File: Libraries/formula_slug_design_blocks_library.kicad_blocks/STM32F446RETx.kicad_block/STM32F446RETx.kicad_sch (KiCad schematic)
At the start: 18 parts

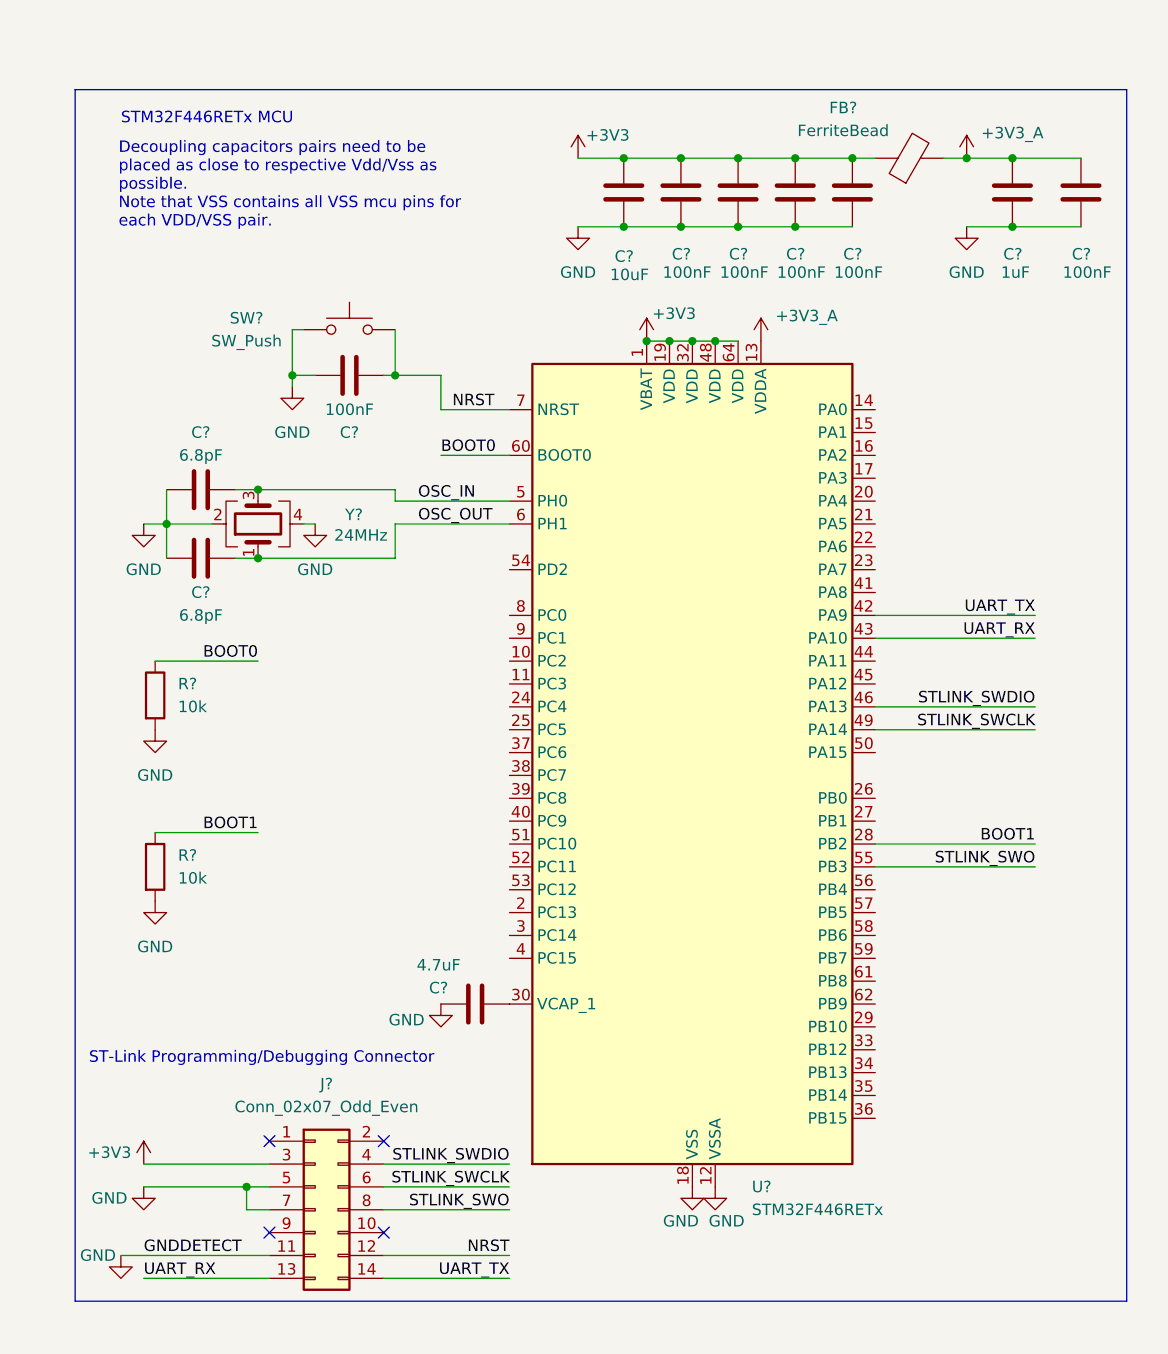
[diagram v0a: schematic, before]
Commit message: Fix issues
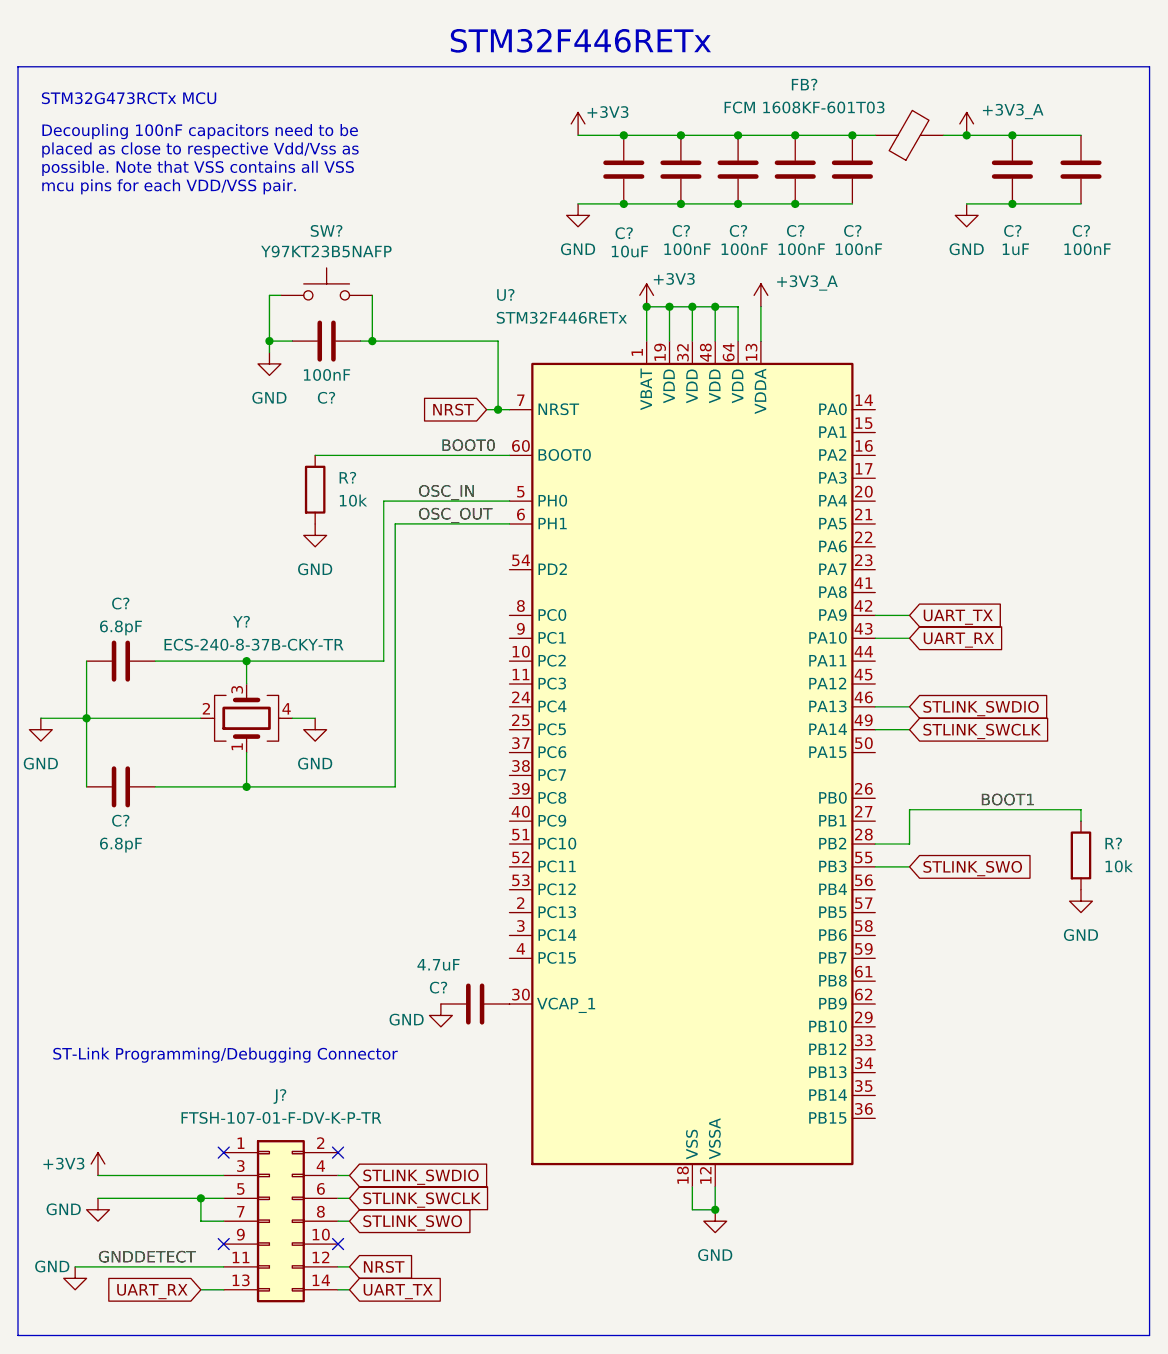
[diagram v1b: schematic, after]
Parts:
- removed C? (x2): 6.8pF, Capacitor_SMD:C_0805_2012Metric_Pad1.18x1.45mm_HandSolder, symbol Device:C
- removed C?: 100nF, Capacitor_SMD:C_0805_2012Metric_Pad1.18x1.45mm_HandSolder, symbol Device:C
- removed J?: Conn_02x07_Odd_Even, Connector_PinHeader_1.27mm:PinHeader_2x07_P1.27mm_Vertical_SMD, symbol Connector_Generic:Conn_02x07_Odd_Even
- removed R?: 10k, Resistor_SMD:R_0805_2012Metric_Pad1.20x1.40mm_HandSolder, symbol Device:R
- removed SW?: SW_Push, Button_Switch_SMD:SW_SPST_PTS647_Sx38, symbol Switch:SW_Push
- removed Y?: 24MHz, Crystal:Crystal_SMD_2016-4Pin_2.0x1.6mm, symbol Device:Crystal_GND24
- added C?: 100nF, Capacitor_SMD:C_0805_2012Metric_Pad1.18x1.45mm_HandSolder, symbol Device:C
- added C? (x2): 6.8pF, Capacitor_SMD:C_0805_2012Metric_Pad1.18x1.45mm_HandSolder, symbol Device:C
- added J?: FTSH-107-01-F-DV-K-P-TR, Connector_PinHeader_1.27mm:PinHeader_2x07_P1.27mm_Vertical_SMD, symbol Connector_Generic:Conn_02x07_Odd_Even
- added R?: 10k, Resistor_SMD:R_0805_2012Metric_Pad1.20x1.40mm_HandSolder, symbol Device:R
- added SW?: Y97KT23B5NAFP, Button_Switch_SMD:SW_SPST_PTS647_Sx38, symbol Switch:SW_Push
- added Y?: ECS-240-8-37B-CKY-TR, Crystal:Crystal_SMD_2016-4Pin_2.0x1.6mm, symbol Device:Crystal_GND24
- C? (x3): Digi URL (none) -> https://www.digikey.com/en/products/detail/samsung-electro-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
- C? (x5): Digi URL (none) -> https://www.digikey.com/en/products/detail/yageo/CC0805KRX7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
- FB?: value FerriteBead -> FCM 1608KF-601T03; Digi URL (none) -> https://www.digikey.com/en/products/detail/tai-tech-advance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
- R?: Digi URL (none) -> https://www.digikey.com/en/products/detail/yageo/AC0805FR-0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
- U?: Digi URL (none) -> https://www.digikey.com/en/products/detail/stmicroelectroni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
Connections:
- net +3V3: now also J?.3 (Pin_3)
- net BOOT1: now also R?.1
- net GND: now also C?.1, C?.2, C?.2, J?.11 (Pin_11), J?.5 (Pin_5), J?.7 (Pin_7), R?.2, SW?.1, Y?.2, Y?.4
- net NRST: now also C?.2, J?.12 (Pin_12), SW?.2
- net OSC_IN: now also C?.1, Y?.3
- net OSC_OUT: now also C?.1, Y?.1
- net STLINK_SWCLK: now also J?.6 (Pin_6)
- net STLINK_SWDIO: now also J?.4 (Pin_4)
- net STLINK_SWO: now also J?.8 (Pin_8)
- net UART_RX: now also J?.13 (Pin_13)
- net UART_TX: now also J?.14 (Pin_14)
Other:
- note added: "Decoupling 100nF capacitors need to be placed as close to respective Vdd/Vss as possible. Note that VSS contains all VSS mcu pins for each VDD/VSS pair."
- note added: "STM32F446RETx"
- note added: "STM32G473RCTx MCU"
- note removed: "Decoupling capacitors pairs need to be placed as close to respective Vdd/Vss as possible. Note that VSS contains all VSS mcu pins for each VDD/VSS pair."
- note removed: "STM32F446RETx MCU"
- moved on the sheet: C?, FB?, R?
